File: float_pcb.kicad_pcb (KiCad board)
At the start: 4 copper layers, 64 x 64 mm, 77 parts, among them J1 Switch, J2 Conn_01x04, J3 USB_C, J4 Conn_01x03, J5 I2C, J6 Light, J7 Batt, J9 I2C, Q1 AO3400A, Q2 AO3400A, U1 TPSM863252, U2 TPSM863252, U3 USBLC6-2SC6, U4 ESP32-S3-WROOM-1, U5 USBLC6-4SC6, U6 USBLC6-4SC6

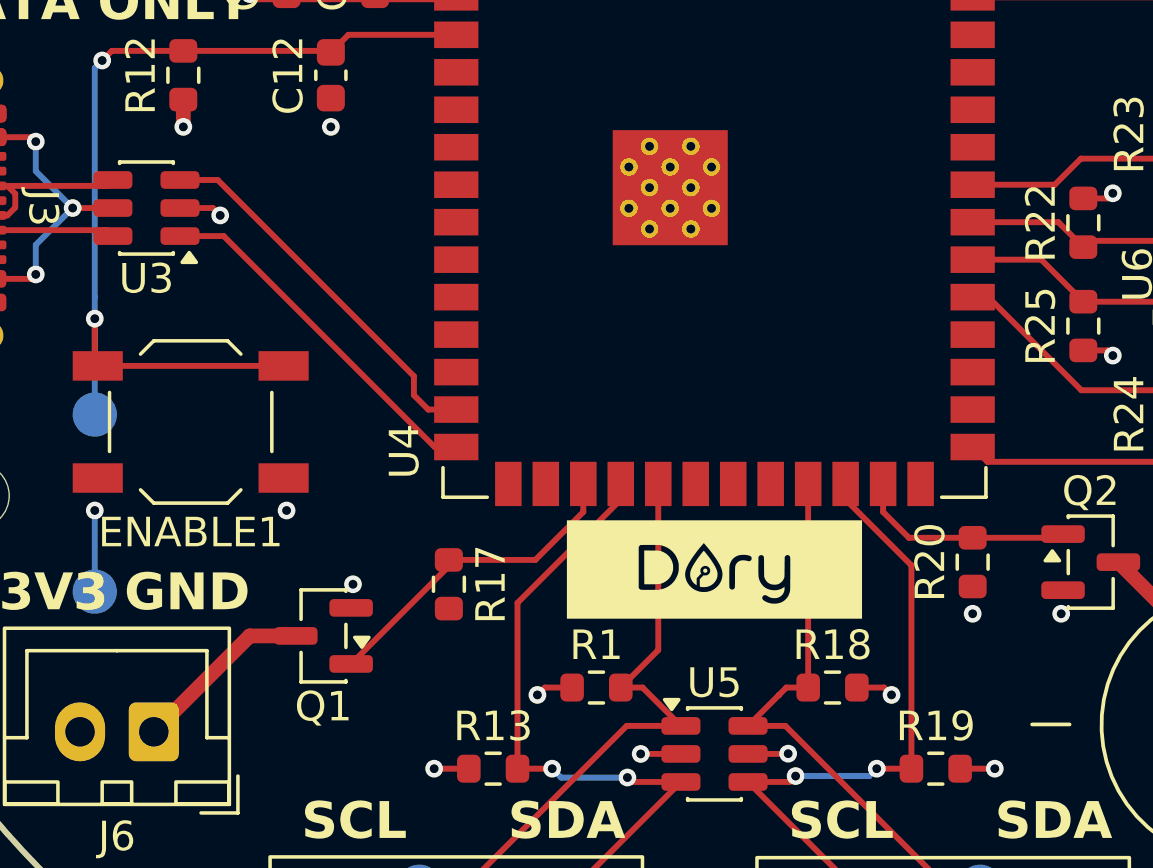
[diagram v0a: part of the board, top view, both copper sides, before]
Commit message: More progress on V4
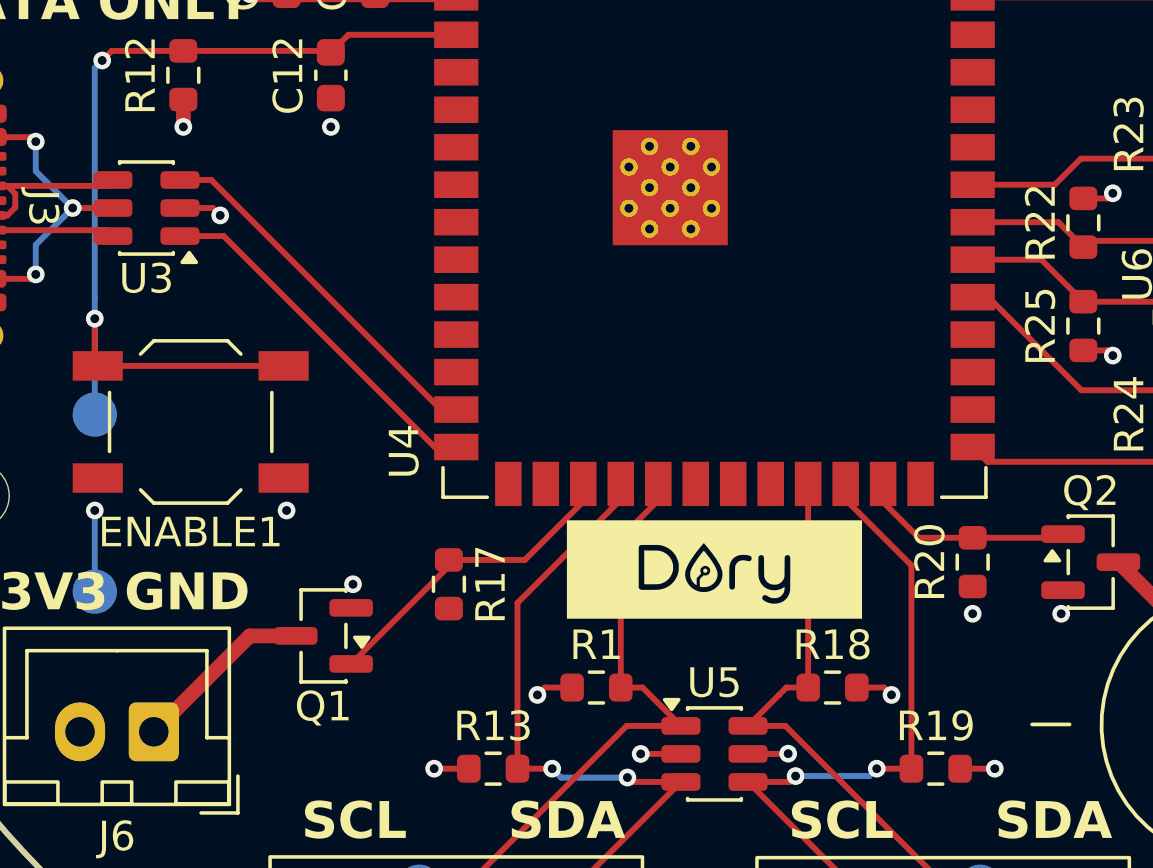
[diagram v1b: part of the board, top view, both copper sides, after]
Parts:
- U4: value ESP32-S3-WROOM-1 -> ESP32-S3-WROOM-1U
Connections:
- net /VBUS renamed VBUS_USB
- net Net-(J3-D+-PadA6) renamed USBC_D+
- net Net-(J3-D--PadA7) renamed USBC_D-
- net Net-(U4-USB_D+) renamed ESP32_D+
- net Net-(U4-USB_D-) renamed ESP32_D-
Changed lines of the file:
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@@
 			)
 		)
-		(property "Value" "ESP32-S3-WROOM-1"
+		(property "Value" "ESP32-S3-WROOM-1U"
 			(at 0 2.46 0)
 			(unlocked yes)
@@
 			(size 1.5 0.9)
 			(layers "F.Cu" "F.Mask" "F.Paste")
-			(net "Net-(U4-USB_D-)")
+			(net "ESP32_D-")
 			(pinfunction "USB_D-_13")
 			(pintype "bidirectional")
@@
 			(size 1.5 0.9)
 			(layers "F.Cu" "F.Mask" "F.Paste")
-			(net "Net-(U4-USB_D+)")
+			(net "ESP32_D+")
 			(pinfunction "USB_D+_14")
 			(pintype "bidirectional")
@@
 			(layers "F.Cu" "F.Mask" "F.Paste")
 			(roundrect_rratio 0.25)
-			(net "/VBUS")
+			(net "VBUS_USB")
 			(pinfunction "VBUS_A4")
 			(pintype "passive")
@@
 			(layers "F.Cu" "F.Mask" "F.Paste")
 			(roundrect_rratio 0.25)
-			(net "Net-(J3-D+-PadA6)")
+			(net "USBC_D+")
 			(pinfunction "D+_A6")
 			(pintype "bidirectional")
@@
 			(layers "F.Cu" "F.Mask" "F.Paste")
 			(roundrect_rratio 0.25)
-			(net "Net-(J3-D--PadA7)")
+			(net "USBC_D-")
 			(pinfunction "D-_A7")
 			(pintype "bidirectional")
@@
 			(layers "F.Cu" "F.Mask" "F.Paste")
 			(roundrect_rratio 0.25)
-			(net "/VBUS")
+			(net "VBUS_USB")
 			(pinfunction "VBUS_A9")
 			(pintype "passive")
@@
 			(layers "F.Cu" "F.Mask" "F.Paste")
 			(roundrect_rratio 0.25)
-			(net "/VBUS")
+			(net "VBUS_USB")
 			(pinfunction "VBUS_B4")
 			(pintype "passive")
@@
 			(layers "F.Cu" "F.Mask" "F.Paste")
 			(roundrect_rratio 0.25)
-			(net "Net-(J3-D+-PadA6)")
+			(net "USBC_D+")
 			(pinfunction "D+_B6")
 			(pintype "bidirectional")
@@
 			(layers "F.Cu" "F.Mask" "F.Paste")
 			(roundrect_rratio 0.25)
-			(net "Net-(J3-D--PadA7)")
+			(net "USBC_D-")
 			(pinfunction "D-_B7")
 			(pintype "bidirectional")
@@
 			(layers "F.Cu" "F.Mask" "F.Paste")
 			(roundrect_rratio 0.25)
-			(net "/VBUS")
+			(net "VBUS_USB")
 			(pinfunction "VBUS_B9")
 			(pintype "passive")
@@
 			(layers "F.Cu" "F.Mask" "F.Paste")
 			(roundrect_rratio 0.25)
-			(net "Net-(U4-USB_D+)")
+			(net "ESP32_D+")
 			(pinfunction "I/O1_1")
 			(pintype "passive")
@@
 			(layers "F.Cu" "F.Mask" "F.Paste")
 			(roundrect_rratio 0.25)
-			(net "Net-(U4-USB_D-)")
+			(net "ESP32_D-")
 			(pinfunction "I/O2_3")
 			(pintype "passive")
@@
 			(layers "F.Cu" "F.Mask" "F.Paste")
 			(roundrect_rratio 0.25)
-			(net "Net-(J3-D--PadA7)")
+			(net "USBC_D-")
 			(pinfunction "I/O2_4")
 			(pintype "passive")
@@
 			(layers "F.Cu" "F.Mask" "F.Paste")
 			(roundrect_rratio 0.25)
-			(net "/VBUS")
+			(net "VBUS_USB")
 			(pinfunction "VBUS_5")
 			(pintype "passive")
@@
 			(layers "F.Cu" "F.Mask" "F.Paste")
 			(roundrect_rratio 0.25)
-			(net "Net-(J3-D+-PadA6)")
+			(net "USBC_D+")
 			(pinfunction "I/O1_6")
 			(pintype "passive")
@@
 	)
 	(segment
-		(start 142.43 116.925)
+		(start 142.075 116.925)
 		(end 139.5 116.925)
 		(width 0.2)
@@
 	)
 	(segment
-		(start 139.5 116.925)
-		(end 139.5 117.1375)
+		(start 144.055 114.35)
+		(end 144.055 114.945)
 		(width 0.2)
 		(layer "F.Cu")
@@
 	)
 	(segment
-		(start 144.055 115.3)
-		(end 142.43 116.925)
+		(start 139.5 116.925)
+		(end 139.5 117.1375)
 		(width 0.2)
 		(layer "F.Cu")
@@
 	)
 	(segment
-		(start 139.5 117.1375)
-		(end 136.1875 120.45)
+		(start 144.055 114.945)
+		(end 142.075 116.925)
 		(width 0.2)
 		(layer "F.Cu")
@@
 	)
 	(segment
-		(start 144.055 114.35)
-		(end 144.055 115.3)
+		(start 139.5 117.1375)
+		(end 136.1875 120.45)
 		(width 0.2)
 		(layer "F.Cu")
@@
 	)
 	(segment
-		(start 146.595 119.98)
+		(start 146.595 114.905)
 		(end 146.595 114.35)
 		(width 0.2)
@@
 	)
 	(segment
+		(start 145.325 116.175)
+		(end 146.595 114.905)
+		(width 0.2)
+		(layer "F.Cu")
+		(net "SCL1")
+	)
+	(segment
 		(start 138.5 130.5)
 		(end 138.5 129.575)
@@
 	(segment
 		(start 145.325 121.25)
-		(end 146.595 119.98)
+		(end 145.325 116.175)
 		(width 0.2)
 		(layer "F.Cu")
@@
 	)
 	(segment
-		(start 157.25 116.175)
-		(end 155.09 116.175)
-		(width 0.2)
-		(layer "F.Cu")
-		(net "BUZZER")
-	)
-	(segment
-		(start 154.215 115.3)
-		(end 154.215 114.35)
+		(start 155.425 116.175)
+		(end 154.215 114.965)
 		(width 0.2)
 		(layer "F.Cu")
@@
 	)
 	(segment
-		(start 155.09 116.175)
-		(end 154.215 115.3)
+		(start 157.25 116.175)
+		(end 155.425 116.175)
 		(width 0.2)
 		(layer "F.Cu")
@@
 	)
 	(segment
-		(start 157.5 80.675)
-		(end 157.5 79.0575)
-		(width 0.2)
-		(layer "F.Cu")
-		(net "Net-(D1-A)")
-	)
-	(segment
-		(start 138.8 111.83)
-		(end 138.314927 111.344927)
+		(start 154.215 114.965)
+		(end 154.215 114.35)
 		(width 0.2)
 		(layer "F.Cu")
-		(net "Net-(U4-USB_D-)")
+		(net "BUZZER")
 	)
 	(segment
-		(start 138.314927 110.698628)
-		(end 131.666299 104.05)
+		(start 157.5 80.675)
+		(end 157.5 79.0575)
 		(width 0.2)
 		(layer "F.Cu")
-		(net "Net-(U4-USB_D-)")
+		(net "Net-(D1-A)")
 	)
 	(segment
-		(start 131.666299 104.05)
-		(end 130.3875 104.05)
+		(start 131.448529 104.05)
+		(end 139.228529 111.83)
 		(width 0.2)
 		(layer "F.Cu")
-		(net "Net-(U4-USB_D-)")
+		(net "ESP32_D-")
 	)
 	(segment
-		(start 138.314927 111.344927)
-		(end 138.314927 110.698628)
+		(start 139.228529 111.83)
+		(end 139.75 111.83)
 		(width 0.2)
 		(layer "F.Cu")
-		(net "Net-(U4-USB_D-)")
+		(net "ESP32_D-")
 	)
 	(segment
-		(start 139.75 111.83)
-		(end 138.8 111.83)
+		(start 130.3875 104.05)
+		(end 131.448529 104.05)
 		(width 0.2)
 		(layer "F.Cu")
-		(net "Net-(U4-USB_D-)")
+		(net "ESP32_D-")
 	)
 	(segment
@@
 		(width 0.2)
 		(layer "F.Cu")
-		(net "Net-(U4-USB_D+)")
+		(net "ESP32_D+")
 	)
 	(segment
@@
 		(width 0.2)
 		(layer "F.Cu")
-		(net "Net-(U4-USB_D+)")
+		(net "ESP32_D+")
 	)
 	(segment
@@
 		(width 0.2)
 		(layer "F.Cu")
-		(net "Net-(U4-USB_D+)")
+		(net "ESP32_D+")
 	)
 	(segment
@@
 		(width 0.2)
 		(layer "F.Cu")
-		(net "/VBUS")
+		(net "VBUS_USB")
 	)
 	(segment
@@
 		(width 0.2)
 		(layer "F.Cu")
-		(net "/VBUS")
+		(net "VBUS_USB")
 	)
 	(segment
@@
 		(width 0.2)
 		(layer "F.Cu")
-		(net "/VBUS")
+		(net "VBUS_USB")
 	)
 	(segment
@@
 		(width 0.2)
 		(layer "F.Cu")
-		(net "/VBUS")
+		(net "VBUS_USB")
 	)
 	(segment
@@
 		(width 0.2)
 		(layer "F.Cu")
-		(net "/VBUS")
+		(net "VBUS_USB")
 	)
 	(via
@@
 		(drill 0.3)
 		(layers "F.Cu" "B.Cu")
-		(net "/VBUS")
+		(net "VBUS_USB")
 	)
 	(via
@@
 		(drill 0.3)
 		(layers "F.Cu" "B.Cu")
-		(net "/VBUS")
+		(net "VBUS_USB")
 	)
 	(via
@@
 		(drill 0.3)
 		(layers "F.Cu" "B.Cu")
-		(net "/VBUS")
+		(net "VBUS_USB")
 	)
 	(segment
@@
 		(width 0.2)
 		(layer "B.Cu")
-		(net "/VBUS")
+		(net "VBUS_USB")
 	)
 	(segment
@@
 		(width 0.2)
 		(layer "B.Cu")
-		(net "/VBUS")
+		(net "VBUS_USB")
 	)
 	(segment
@@
 		(width 0.2)
 		(layer "B.Cu")
-		(net "/VBUS")
+		(net "VBUS_USB")
 	)
 	(segment
@@
 		(width 0.2)
 		(layer "B.Cu")
-		(net "/VBUS")
+		(net "VBUS_USB")
 	)
 	(segment
@@
 		(width 0.2)
 		(layer "F.Cu")
-		(net "Net-(J3-D+-PadA6)")
+		(net "USBC_D+")
 	)
 	(segment
@@
 		(width 0.2)
 		(layer "F.Cu")
-		(net "Net-(J3-D+-PadA6)")
+		(net "USBC_D+")
 	)
 	(segment
@@
 		(width 0.2)
 		(layer "F.Cu")
-		(net "Net-(J3-D+-PadA6)")
+		(net "USBC_D+")
 	)
 	(segment
@@
 		(width 0.2)
 		(layer "F.Cu")
-		(net "Net-(J3-D+-PadA6)")
+		(net "USBC_D+")
 	)
 	(segment
@@
 		(width 0.2)
 		(layer "F.Cu")
-		(net "Net-(J3-D+-PadA6)")
+		(net "USBC_D+")
 	)
 	(segment
@@
 		(width 0.2)
 		(layer "F.Cu")
-		(net "Net-(J3-D+-PadA6)")
+		(net "USBC_D+")
 	)
 	(segment
@@
 		(width 0.2)
 		(layer "F.Cu")
-		(net "Net-(J3-D+-PadA6)")
+		(net "USBC_D+")
 	)
 	(segment
@@
 		(width 0.2)
 		(layer "F.Cu")
-		(net "Net-(J3-D--PadA7)")
+		(net "USBC_D-")
 	)
 	(segment
@@
 		(width 0.2)
 		(layer "F.Cu")
-		(net "Net-(J3-D--PadA7)")
+		(net "USBC_D-")
 	)
 	(segment
@@
 		(width 0.2)
 		(layer "F.Cu")
-		(net "Net-(J3-D--PadA7)")
+		(net "USBC_D-")
 	)
 	(segment
@@
 		(width 0.2)
 		(layer "F.Cu")
-		(net "Net-(J3-D--PadA7)")
+		(net "USBC_D-")
 	)
 	(segment
@@
 		(width 0.2)
 		(layer "F.Cu")
-		(net "Net-(J3-D--PadA7)")
+		(net "USBC_D-")
 	)
 	(segment
@@
 		(width 0.2)
 		(layer "F.Cu")
-		(net "Net-(J3-D--PadA7)")
+		(net "USBC_D-")
 	)
 	(segment
@@
 		(width 0.2)
 		(layer "F.Cu")
-		(net "Net-(J3-D--PadA7)")
+		(net "USBC_D-")
 	)
 	(zone
